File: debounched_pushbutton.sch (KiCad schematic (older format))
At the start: 4 parts, among them SW1 SW_Push_Dual

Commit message: joo
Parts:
- SW1: footprint Button_Switch_THT:SW_PUSH_6mm -> Button_Switch_THT:SW_Tactile_Straight_KSA0Axx1LFTR
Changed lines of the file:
@@
 $Descr A4 11693 8268
 encoding utf-8
-Sheet 7 8
+Sheet 22 22
 Title ""
 Date ""
@@
 F 0 "SW2" H 1450 1635 50  0000 C CNN
 F 1 "SW_Push_Dual" H 1450 1544 50  0000 C CNN
-F 2 "Button_Switch_THT:SW_PUSH_6mm" H 1450 1550 50  0001 C CNN
+F 2 "Button_Switch_THT:SW_Tactile_Straight_KSA0Axx1LFTR" H 1450 1550 50  0001 C CNN
 F 3 "" H 1450 1550 50  0001 C CNN
 	1    1450 1350

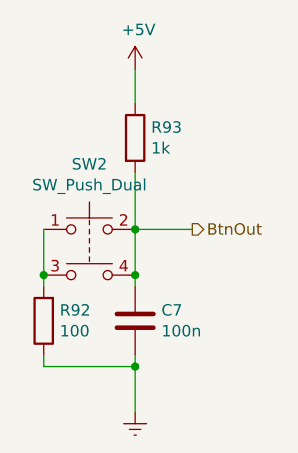
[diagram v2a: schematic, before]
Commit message: nonni
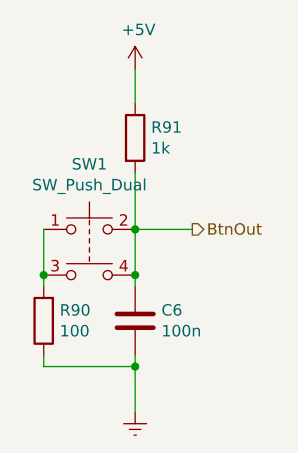
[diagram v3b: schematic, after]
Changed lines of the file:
@@
 AR Path="/5E7FE069/5E804E14" Ref="SW1"  Part="1"
 AR Path="/5E8135E4/5E804E14" Ref="SW2"  Part="1"
-F 0 "SW2" H 1450 1635 50  0000 C CNN
+F 0 "SW1" H 1450 1635 50  0000 C CNN
 F 1 "SW_Push_Dual" H 1450 1544 50  0000 C CNN
 F 2 "Button_Switch_THT:SW_Tactile_Straight_KSA0Axx1LFTR" H 1450 1550 50  0001 C CNN
@@
 AR Path="/5E7FE069/5E804E1C" Ref="R91"  Part="1"
 AR Path="/5E8135E4/5E804E1C" Ref="R93"  Part="1"
-F 0 "R93" H 1720 996 50  0000 L CNN
+F 0 "R91" H 1720 996 50  0000 L CNN
 F 1 "1k" H 1720 905 50  0000 L CNN
 F 2 "Resistor_SMD:R_0805_2012Metric" V 1580 950 50  0001 C CNN
@@
 AR Path="/5E7FE069/5E804E22" Ref="R90"  Part="1"
 AR Path="/5E8135E4/5E804E22" Ref="R92"  Part="1"
-F 0 "R92" H 1180 1704 50  0000 R CNN
+F 0 "R90" H 1180 1704 50  0000 R CNN
 F 1 "100" H 1180 1795 50  0000 R CNN
 F 2 "Resistor_SMD:R_0805_2012Metric" V 1180 1750 50  0001 C CNN
@@
 AR Path="/5E7FE069/5E804E2C" Ref="C6"  Part="1"
 AR Path="/5E8135E4/5E804E2C" Ref="C7"  Part="1"
-F 0 "C7" H 1535 1704 50  0000 R CNN
+F 0 "C6" H 1535 1704 50  0000 R CNN
 F 1 "100n" H 1535 1795 50  0000 R CNN
 F 2 "Capacitor_SMD:C_0805_2012Metric" H 1688 1600 50  0001 C CNN

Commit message: tilasin nää
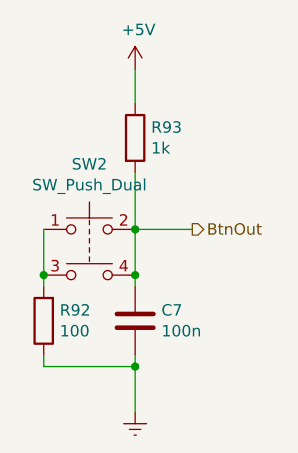
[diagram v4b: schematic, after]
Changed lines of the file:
@@
 AR Path="/5E7FE069/5E804E14" Ref="SW1"  Part="1"
 AR Path="/5E8135E4/5E804E14" Ref="SW2"  Part="1"
-F 0 "SW1" H 1450 1635 50  0000 C CNN
+F 0 "SW2" H 1450 1635 50  0000 C CNN
 F 1 "SW_Push_Dual" H 1450 1544 50  0000 C CNN
 F 2 "Button_Switch_THT:SW_Tactile_Straight_KSA0Axx1LFTR" H 1450 1550 50  0001 C CNN
@@
 AR Path="/5E7FE069/5E804E1C" Ref="R91"  Part="1"
 AR Path="/5E8135E4/5E804E1C" Ref="R93"  Part="1"
-F 0 "R91" H 1720 996 50  0000 L CNN
+F 0 "R93" H 1720 996 50  0000 L CNN
 F 1 "1k" H 1720 905 50  0000 L CNN
 F 2 "Resistor_SMD:R_0805_2012Metric" V 1580 950 50  0001 C CNN
@@
 AR Path="/5E7FE069/5E804E22" Ref="R90"  Part="1"
 AR Path="/5E8135E4/5E804E22" Ref="R92"  Part="1"
-F 0 "R90" H 1180 1704 50  0000 R CNN
+F 0 "R92" H 1180 1704 50  0000 R CNN
 F 1 "100" H 1180 1795 50  0000 R CNN
 F 2 "Resistor_SMD:R_0805_2012Metric" V 1180 1750 50  0001 C CNN
@@
 AR Path="/5E7FE069/5E804E2C" Ref="C6"  Part="1"
 AR Path="/5E8135E4/5E804E2C" Ref="C7"  Part="1"
-F 0 "C6" H 1535 1704 50  0000 R CNN
+F 0 "C7" H 1535 1704 50  0000 R CNN
 F 1 "100n" H 1535 1795 50  0000 R CNN
 F 2 "Capacitor_SMD:C_0805_2012Metric" H 1688 1600 50  0001 C CNN
